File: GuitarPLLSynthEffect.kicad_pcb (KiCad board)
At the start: 2 copper layers, 183.9 x 110 mm, 75 parts

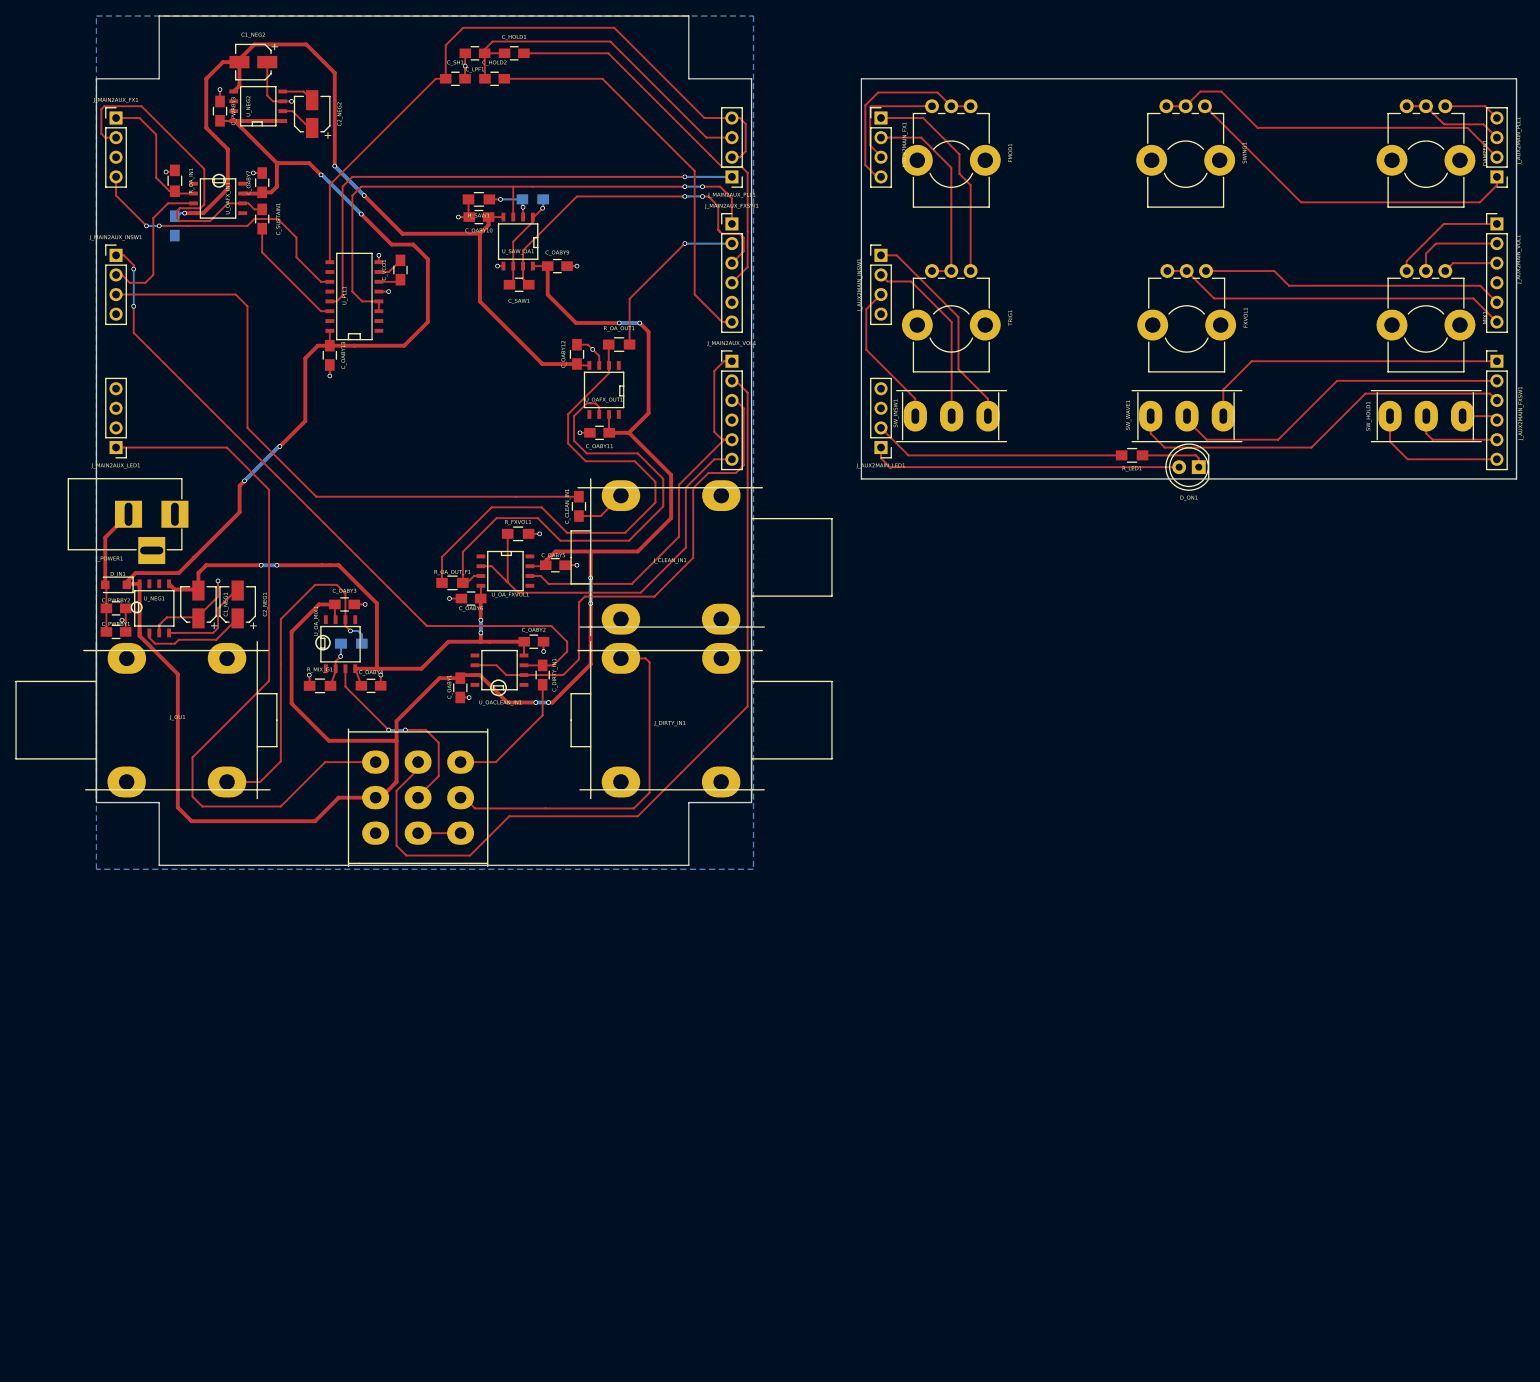
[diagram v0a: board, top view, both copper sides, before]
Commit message: Second draft PCB layout
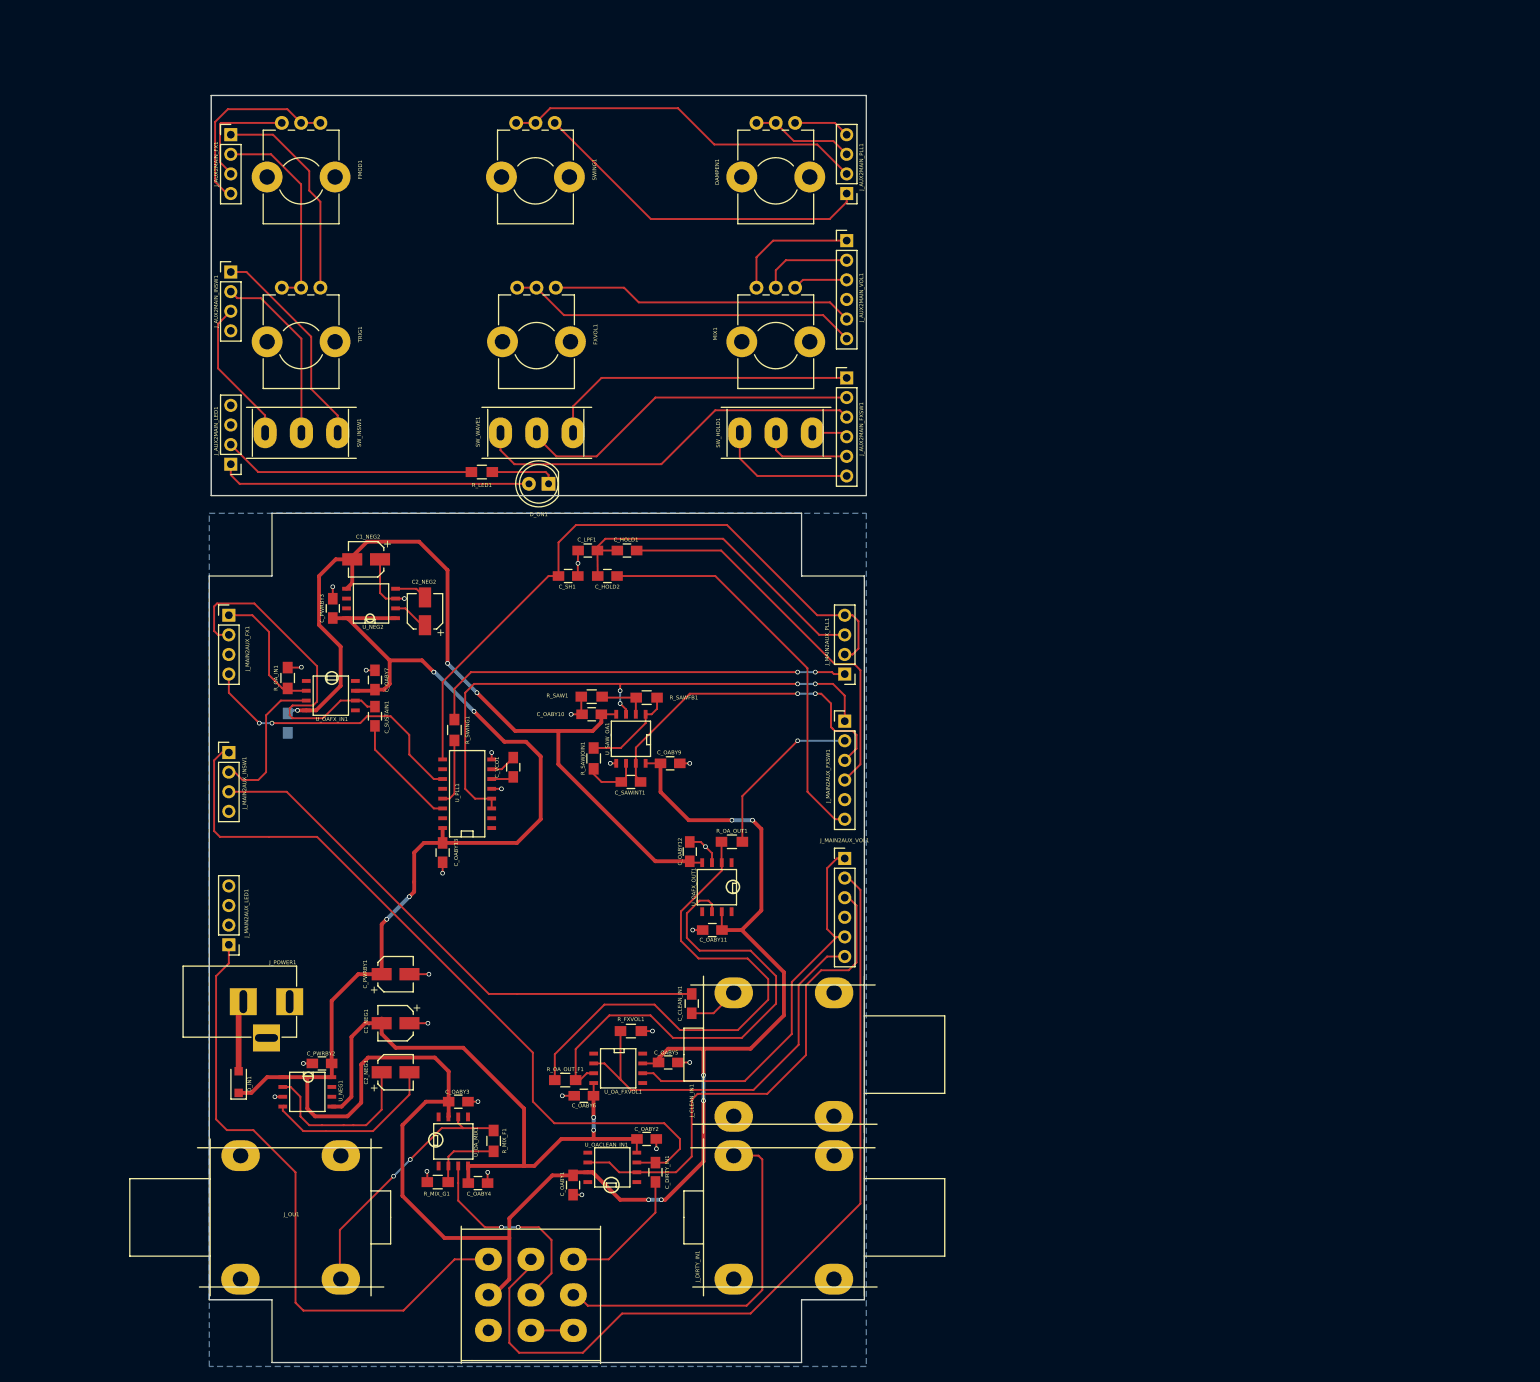
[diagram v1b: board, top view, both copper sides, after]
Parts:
- removed C_SAW1: 10nF, Capacitors_SMD:C_0805_HandSoldering
- removed R_SAW2: 1K, Resistors_SMD:R_0805_HandSoldering
- added C_SAWINT1: 10nF, Capacitors_SMD:C_0805_HandSoldering, F.Cu at (112.4, 142.4)
- added R_SAWFB1: 1K, Resistors_SMD:R_0805_HandSoldering, F.Cu at (114.4, 131.4)
- added R_SAWJOIN1: 10R, Resistors_SMD:R_0805_HandSoldering, F.Cu at (107.6, 139.3)
- added R_SWING1: 22K, Resistors_SMD:R_0805_HandSoldering, F.Cu at (89.5, 135.6)
- C_PWRBY1: footprint Capacitors_SMD:C_0805_HandSoldering -> Capacitors_SMD:CP_Elec_4x5.3
- R_MIX_F1: moved to F.Cu
- moved FXVOL1 84.2 mm to (97.7, 78.4)
- moved R_LED1 84.2 mm to (93.1, 102.2)
- moved SW_INSW1 84.2 mm to (69.7, 97.2)
- moved DAMPEN1 84.2 mm to (128.7, 57.0)
- moved D_ON1 84.2 mm to (101.7, 103.8)
- moved J_AUX2MAIN_FX1 84.2 mm to (60.6, 58.5)
- moved J_AUX2MAIN_FXSW1 84.2 mm to (140.3, 90.0)
- moved J_AUX2MAIN_INSW1 84.2 mm to (60.6, 76.3)
- moved J_AUX2MAIN_LED1 84.2 mm to (60.6, 101.2)
- moved J_AUX2MAIN_PLL1 84.2 mm to (140.3, 66.2)
- moved J_AUX2MAIN_VOL1 84.2 mm to (140.3, 72.3)
- moved MIX1 84.2 mm to (128.7, 78.4)
- moved SWING1 84.2 mm to (97.5, 57.0)
- moved SW_HOLD1 84.2 mm to (131.2, 97.2)
- moved SW_WAVE1 84.2 mm to (100.2, 97.2)
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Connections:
- C_PWRBY1 pad 1: Net-(C_PWRBY1-Pad1) -> /9V
- C_PWRBY2 pad 2: Net-(C_PWRBY1-Pad1) -> /9V
- D_IN1 pad 2: Net-(C_PWRBY1-Pad1) -> Net-(D_IN1-Pad2)
- J_POWER1 pad 2: Net-(C_PWRBY1-Pad1) -> Net-(D_IN1-Pad2)
- U_PLL1 pad 13: /Sheet5AC1BF71/SWING_P3 -> Net-(R_SWING1-Pad2)
- U_SAW_OA1 pad 1: Net-(C_SAW1-Pad2) -> Net-(R_SAWFB1-Pad1)
- U_SAW_OA1 pad 6: Net-(C_SAW1-Pad2) -> Net-(C_SAWINT1-Pad2)
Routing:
- net /9V: track 344.7 -> 325.8 mm
- net Net-(C_PWRBY1-Pad1): track 16.6 -> 0.00 mm
- net Net-(C_SAW1-Pad2): track 12.9 -> 0.00 mm, vias 1 -> 0
- net Net-(R_SAWFB1-Pad1): track 0.00 -> 12.6 mm
- net Net-(D_IN1-Pad2): track 0.00 -> 11.9 mm
- net /Sheet5AC1BF71/SWING_P3: track 67.0 -> 55.5 mm, vias 1 -> 2
- net Net-(J_OU1-Pad1): track 45.1 -> 33.7 mm, vias 1 -> 2
- net /LED_ANODE: track 92.5 -> 81.5 mm
- net Net-(C2_NEG1-Pad2): track 12.6 -> 23.6 mm
- net /INSW_P3: track 80.0 -> 70.8 mm
- net Net-(C2_NEG1-Pad1): track 13.7 -> 22.6 mm
- net Net-(R_SWING1-Pad2): track 0.00 -> 8.69 mm
- net /GND: track 57.7 -> 49.6 mm, vias 23 -> 25
- net /-9V: track 75.4 -> 82.8 mm, vias 4 -> 2
- net Net-(C_SAWINT1-Pad2): track 0.00 -> 7.29 mm
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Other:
- board size 183.9 x 110 mm -> 85.1 x 164.1 mm
